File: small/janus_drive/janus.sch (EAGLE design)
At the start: 28 parts, among them IC1 LM741

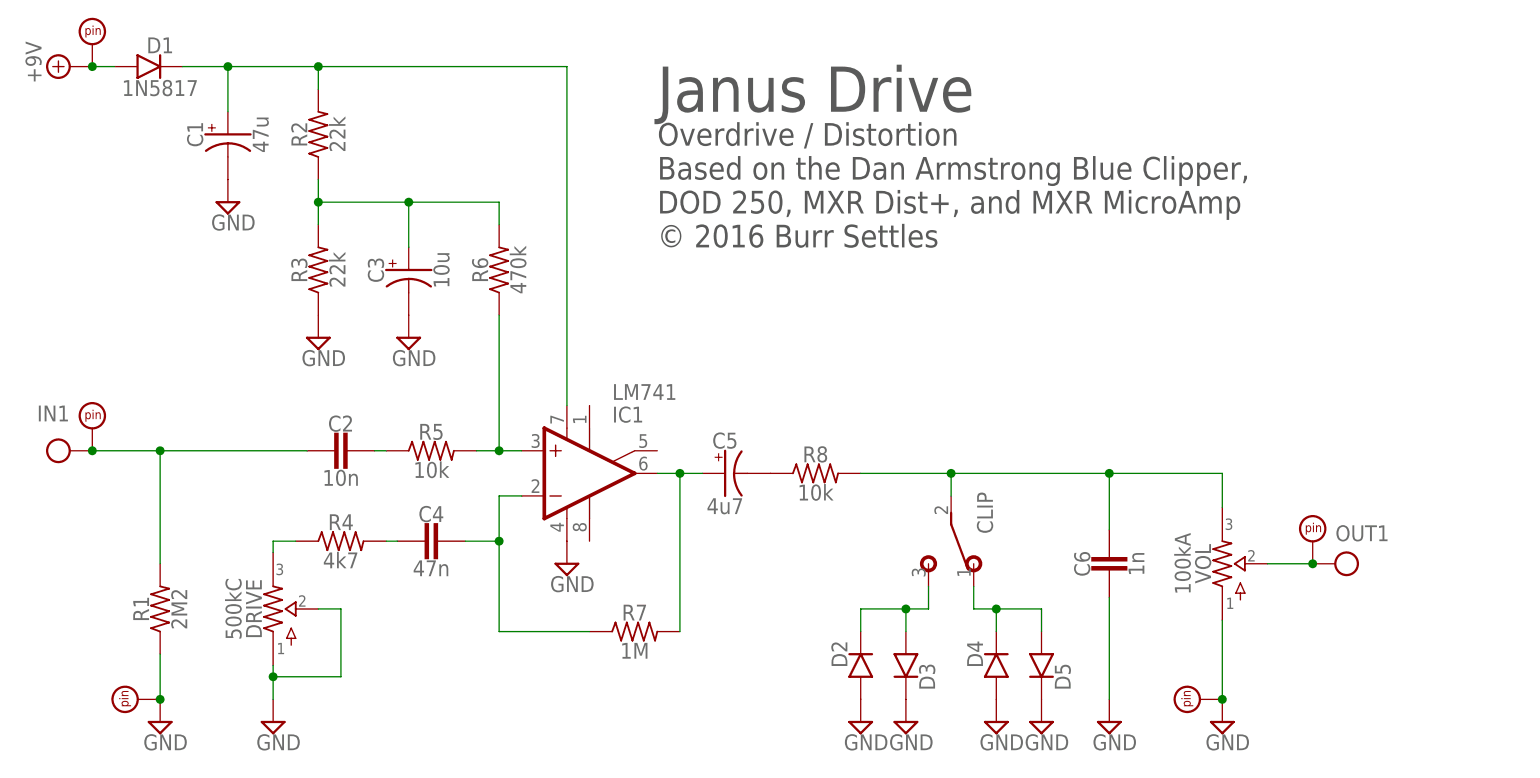
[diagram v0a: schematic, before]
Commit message: updates to a few small pedals
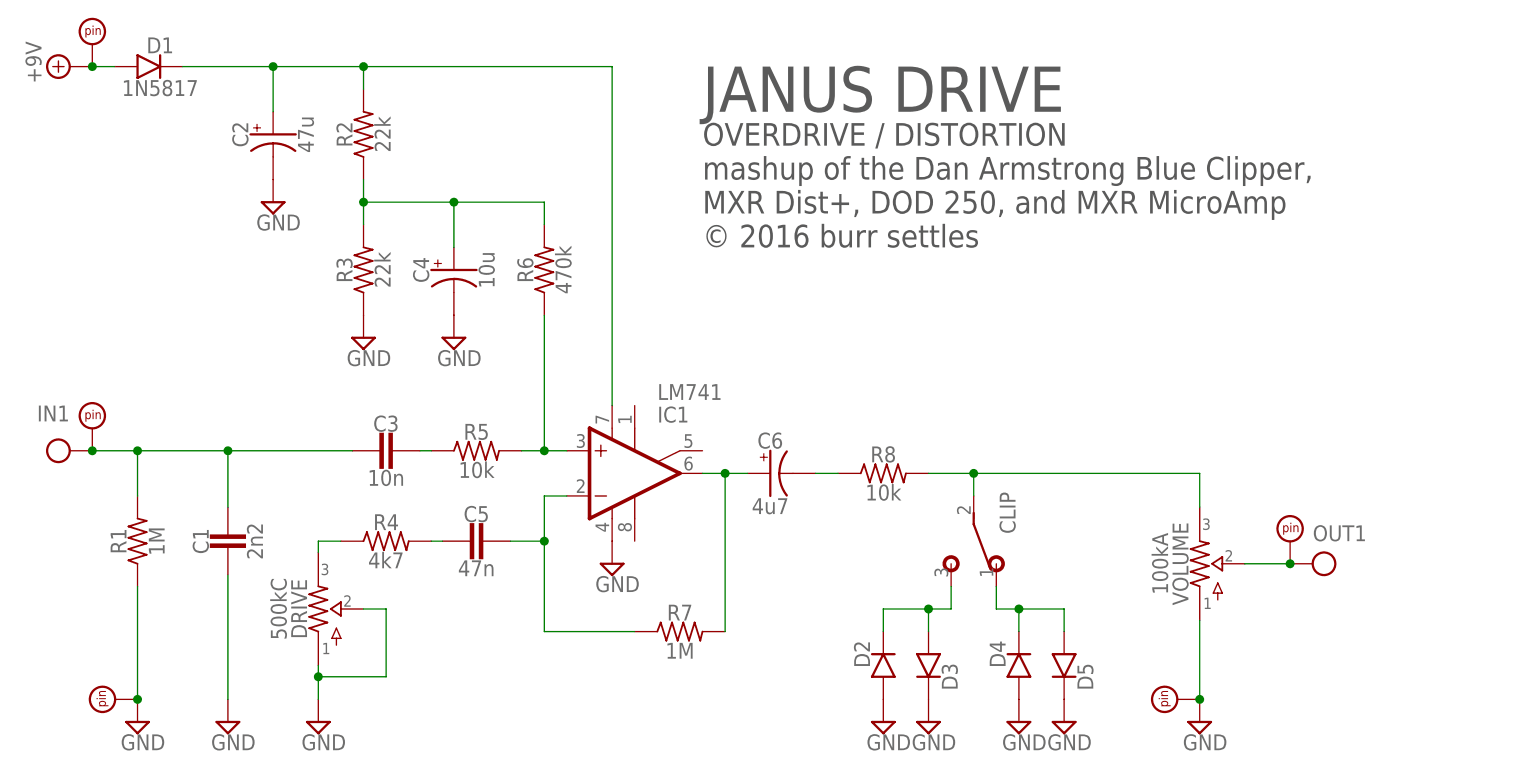
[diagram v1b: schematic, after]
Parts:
- removed VOL: 100kA, potentiometers:POTSSMALL_PADS
- added VOLUME: 100kA, potentiometers:POTSSMALL_PADS
- C1: value 47u -> 2n2; device capacitors-elec:0501 -> capacitors-film:CER/FILMBOX.1
- C2: value 10n -> 47u; device capacitors-film:CER/FILMBOX.1 -> capacitors-elec:0501
- C3: value 10u -> 10n; device capacitors-elec:0501 -> capacitors-film:CER/FILMBOX.1
- C4: value 47n -> 10u; device capacitors-film:CER/FILMBOX.1 -> capacitors-elec:0501
- C5: value 4u7 -> 47n; device capacitors-elec:0501 -> capacitors-film:CER/FILMBOX.1
- C6: value 1n -> 4u7; device capacitors-film:CER/FILMBOX.1 -> capacitors-elec:0501
- R1: value 2M2 -> 1M
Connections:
- net CLIP: now also VOLUME.3; no longer C6.2, VOL.3
- net GND: now also C1.1, C2.-, C4.-, VOLUME.1; no longer C1.-, C3.-, C6.1, VOL.1
- net IN: now also C1.2, C3.2; no longer C2.2
- net N$1: now also C3.1; no longer C2.1
- net N$12: now also C2.+; no longer C1.+
- net N$3: now also C5.1; no longer C4.1
- net N$4: now also C5.2; no longer C4.2
- net N$5: now also C6.+; no longer C5.+
- net N$6: now also C6.-; no longer C5.-
- net N$8: now also C4.+; no longer C3.+
- net OUT: now also VOLUME.2; no longer VOL.2
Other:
- note added: "JANUS DRIVE"
- note added: "OVERDRIVE / DISTORTION mashup of the Dan Armstrong Blue Clipper, MXR Dist+, DOD 250, and MXR MicroAmp © 2016 burr settles"
- note removed: "Janus Drive"
- note removed: "Overdrive / Distortion Based on the Dan Armstrong Blue Clipper, DOD 250, MXR Dist+, and MXR MicroAmp © 2016 Burr Settles"
- moved on the sheet: CLIP, D2, D3, D4, D5, DRIVE, IC1, R1, R2, R3, R4, R5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
